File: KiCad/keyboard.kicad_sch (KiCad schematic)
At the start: 120 parts, among them J1 OLED_128x32, J2 Conn_01x02_Socket, J3 4P4C, J4 OLED_128x32, J5 Conn_01x02_Socket, J6 4P4C, SW1 Switch, SW2 SW_SPDT, SW3 Switch, SW4 SW_SPDT, U1 XIAO-HALF-HOLE-23P, U3 XIAO-HALF-HOLE-23P

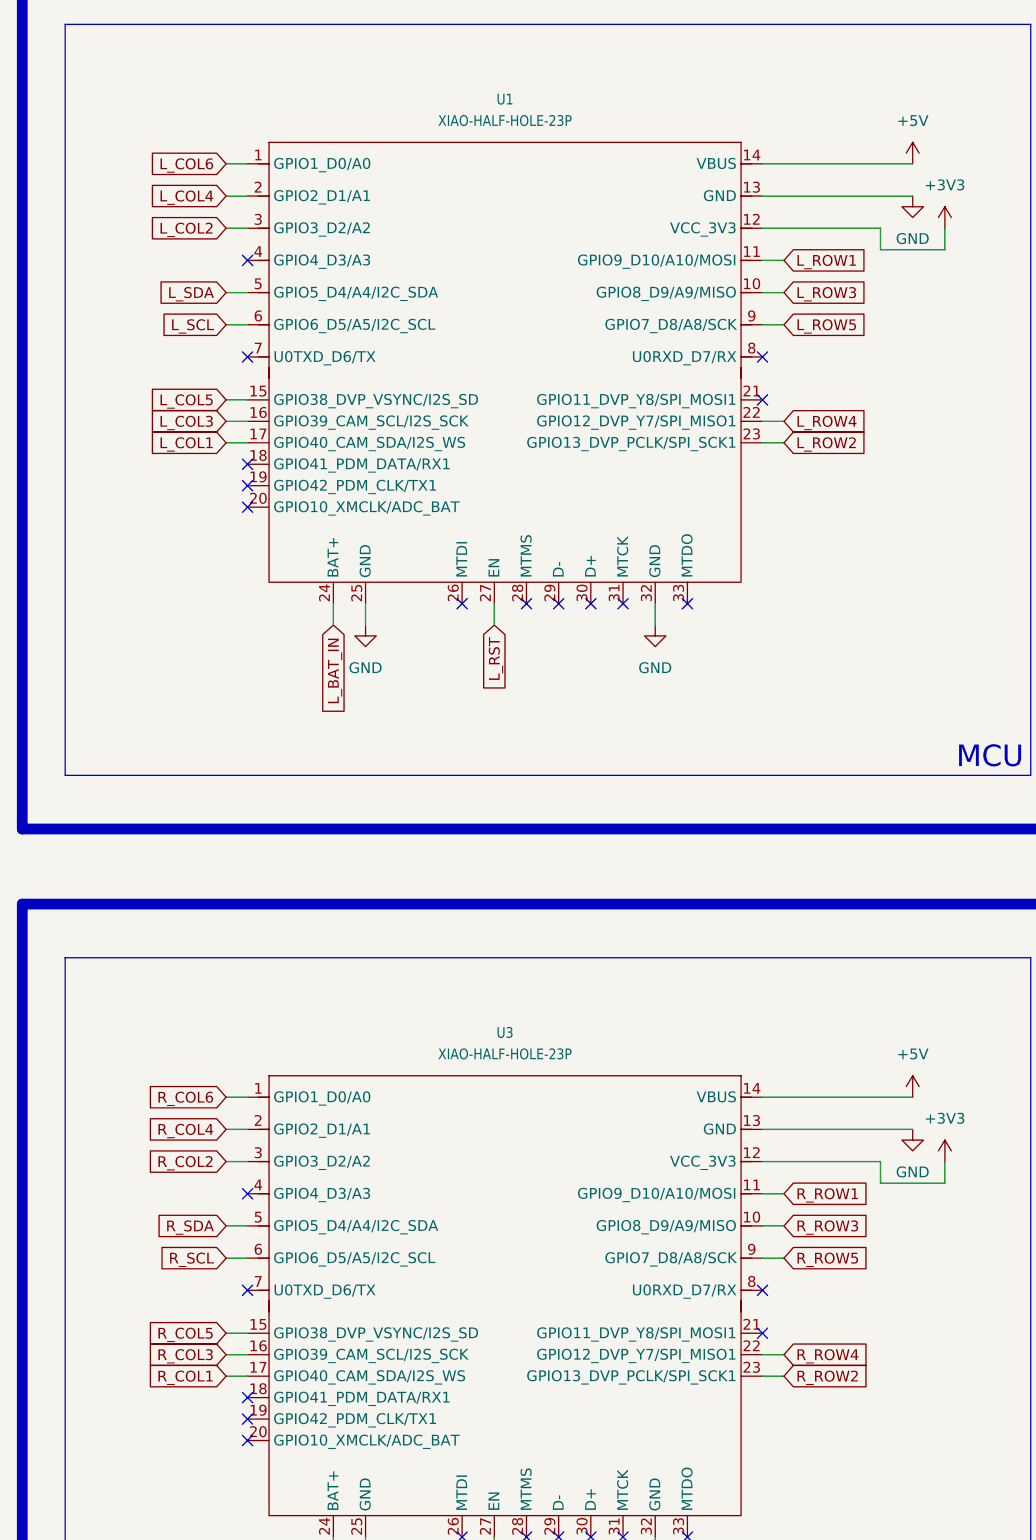
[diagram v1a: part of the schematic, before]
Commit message: PCB
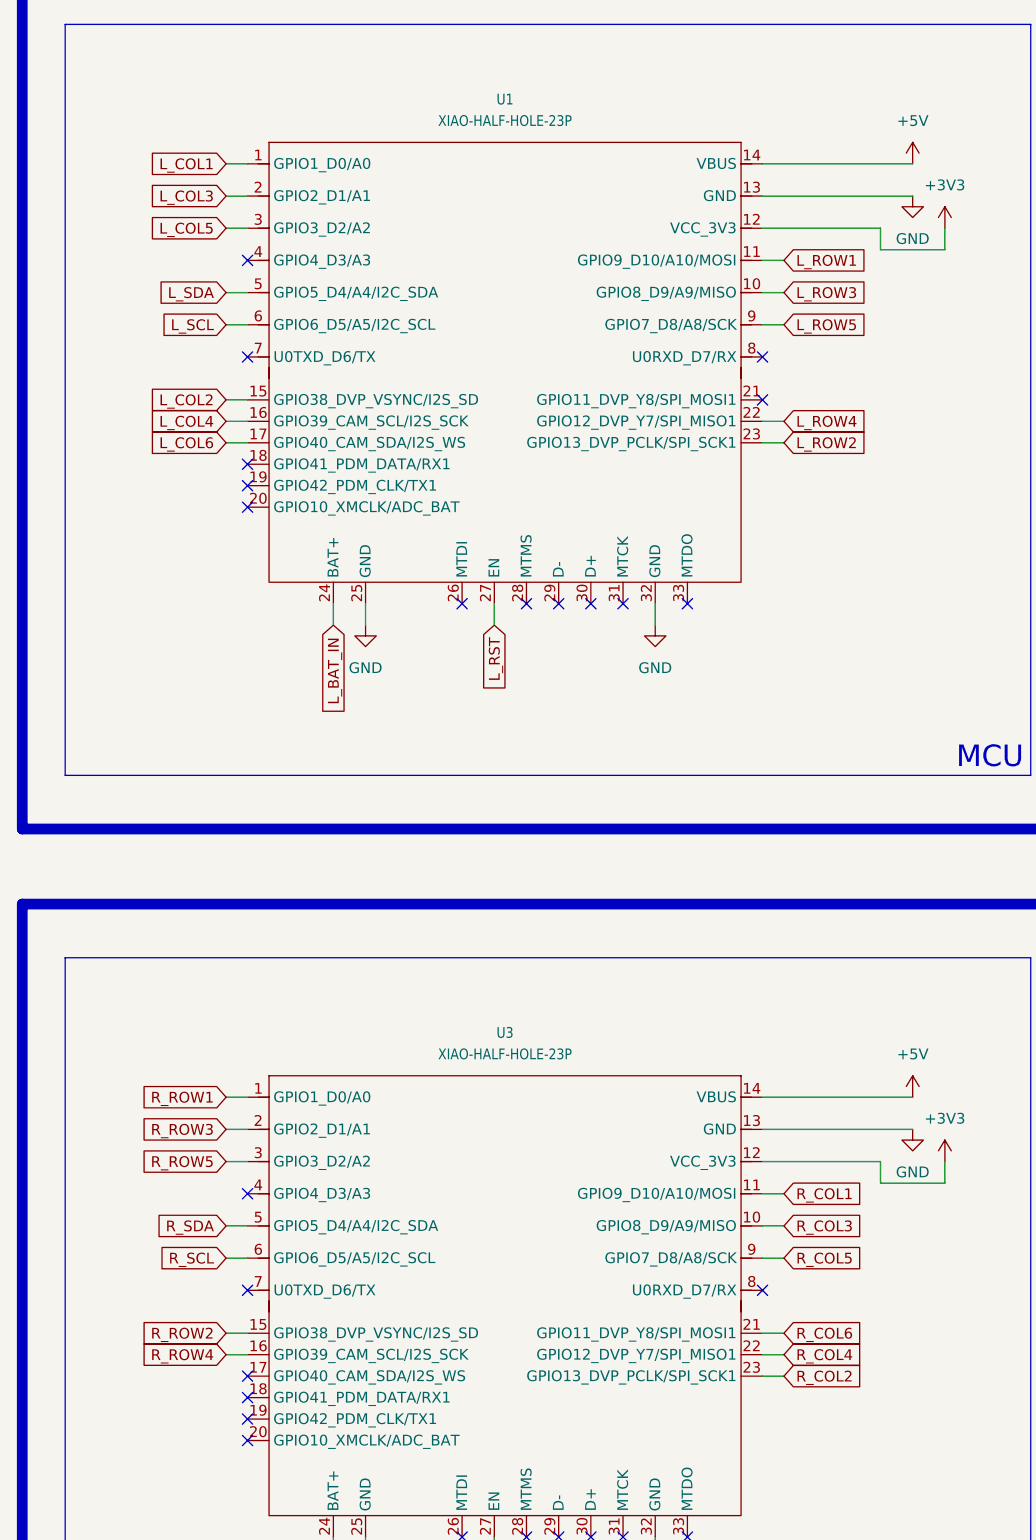
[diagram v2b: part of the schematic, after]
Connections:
- net L_COL1: now also U1.1 (GPIO1_D0/A0); no longer U1.17 (GPIO40_CAM_SDA/I2S_WS)
- net L_COL2: now also U1.15 (GPIO38_DVP_VSYNC/I2S_SD); no longer U1.3 (GPIO3_D2/A2)
- net L_COL3: now also U1.2 (GPIO2_D1/A1); no longer U1.16 (GPIO39_CAM_SCL/I2S_SCK)
- net L_COL4: now also U1.16 (GPIO39_CAM_SCL/I2S_SCK); no longer U1.2 (GPIO2_D1/A1)
- net L_COL5: now also U1.3 (GPIO3_D2/A2); no longer U1.15 (GPIO38_DVP_VSYNC/I2S_SD)
- net L_COL6: now also U1.17 (GPIO40_CAM_SDA/I2S_WS); no longer U1.1 (GPIO1_D0/A0)
- net R_COL1: now also U3.11 (GPIO9_D10/A10/MOSI); no longer U3.17 (GPIO40_CAM_SDA/I2S_WS)
- net R_COL2: now also U3.23 (GPIO13_DVP_PCLK/SPI_SCK1); no longer U3.3 (GPIO3_D2/A2)
- net R_COL3: now also U3.10 (GPIO8_D9/A9/MISO); no longer U3.16 (GPIO39_CAM_SCL/I2S_SCK)
- net R_COL4: now also U3.22 (GPIO12_DVP_Y7/SPI_MISO1); no longer U3.2 (GPIO2_D1/A1)
- net R_COL5: now also U3.9 (GPIO7_D8/A8/SCK); no longer U3.15 (GPIO38_DVP_VSYNC/I2S_SD)
- net R_COL6: now also U3.21 (GPIO11_DVP_Y8/SPI_MOSI1); no longer U3.1 (GPIO1_D0/A0)
- net R_ROW1: now also U3.1 (GPIO1_D0/A0); no longer U3.11 (GPIO9_D10/A10/MOSI)
- net R_ROW2: now also U3.15 (GPIO38_DVP_VSYNC/I2S_SD); no longer U3.23 (GPIO13_DVP_PCLK/SPI_SCK1)
- net R_ROW3: now also U3.2 (GPIO2_D1/A1); no longer U3.10 (GPIO8_D9/A9/MISO)
- net R_ROW4: now also U3.16 (GPIO39_CAM_SCL/I2S_SCK); no longer U3.22 (GPIO12_DVP_Y7/SPI_MISO1)
- net R_ROW5: now also U3.3 (GPIO3_D2/A2); no longer U3.9 (GPIO7_D8/A8/SCK)
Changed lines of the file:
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@@
 	)
 	(no_connect
-		(at 125.73 195.58)
-	)
-	(no_connect
 		(at 64.77 203.2)
 	)
@@
 	)
 	(no_connect
+		(at 64.77 200.66)
+	)
+	(no_connect
 		(at 64.77 208.28)
 	)
@@
 	(wire
 		(pts
-			(xy 62.23 200.66) (xy 64.77 200.66)
-		)
-		(stroke
-			(width 0)
-			(type default)
-		)
-	)
-	(wire
-		(pts
 			(xy 311.15 220.98) (xy 323.85 220.98)
 		)
@@
 	(wire
 		(pts
+			(xy 128.27 195.58) (xy 125.73 195.58)
+		)
+		(stroke
+			(width 0)
+			(type default)
+		)
+	)
+	(wire
+		(pts
 			(xy 280.67 172.72) (xy 280.67 185.42)
 		)
@@
 	(global_label "R_COL6"
 		(shape input)
-		(at 62.23 167.64 180)
+		(at 128.27 195.58 0)
 		(fields_autoplaced yes)
 		(effects
@@
 				(size 1.27 1.27)
 			)
-			(justify right)
+			(justify left)
 		)
 		(property "Intersheetrefs" "${INTERSHEET_REFS}"
-			(at 52.1691 167.64 0)
+			(at 138.3309 195.58 0)
 			(effects
 				(font
 					(size 1.27 1.27)
 				)
-				(justify right)
+				(justify left)
 				(hide yes)
 			)
@@
 	(global_label "L_COL5"
 		(shape input)
-		(at 62.23 85.09 180)
+		(at 62.23 64.77 180)
 		(fields_autoplaced yes)
 		(effects
@@
 		)
 		(property "Intersheetrefs" "${INTERSHEET_REFS}"
-			(at 52.411 85.09 0)
+			(at 52.411 64.77 0)
 			(effects
 				(font
@@
 	(global_label "R_COL3"
 		(shape input)
-		(at 62.23 198.12 180)
+		(at 128.27 182.88 0)
 		(fields_autoplaced yes)
 		(effects
@@
 				(size 1.27 1.27)
 			)
-			(justify right)
+			(justify left)
 		)
 		(property "Intersheetrefs" "${INTERSHEET_REFS}"
-			(at 52.1691 198.12 0)
+			(at 138.3309 182.88 0)
 			(effects
 				(font
 					(size 1.27 1.27)
 				)
-				(justify right)
+				(justify left)
 				(hide yes)
 			)
@@
 	(global_label "R_ROW2"
 		(shape input)
-		(at 128.27 200.66 0)
+		(at 62.23 195.58 180)
 		(fields_autoplaced yes)
 		(effects
@@
 				(size 1.27 1.27)
 			)
-			(justify left)
+			(justify right)
 		)
 		(property "Intersheetrefs" "${INTERSHEET_REFS}"
-			(at 138.7542 200.66 0)
+			(at 51.7458 195.58 0)
 			(effects
 				(font
 					(size 1.27 1.27)
 				)
-				(justify left)
+				(justify right)
 				(hide yes)
 			)
@@
 	(global_label "L_COL1"
 		(shape input)
-		(at 62.23 90.17 180)
+		(at 62.23 57.15 180)
 		(fields_autoplaced yes)
 		(effects
@@
 		)
 		(property "Intersheetrefs" "${INTERSHEET_REFS}"
-			(at 52.411 90.17 0)
+			(at 52.411 57.15 0)
 			(effects
 				(font
@@
 	(global_label "L_COL3"
 		(shape input)
-		(at 62.23 87.63 180)
+		(at 62.23 60.96 180)
 		(fields_autoplaced yes)
 		(effects
@@
 		)
 		(property "Intersheetrefs" "${INTERSHEET_REFS}"
-			(at 52.411 87.63 0)
+			(at 52.411 60.96 0)
 			(effects
 				(font
@@
 	(global_label "R_COL5"
 		(shape input)
-		(at 62.23 195.58 180)
+		(at 128.27 186.69 0)
 		(fields_autoplaced yes)
 		(effects
@@
 				(size 1.27 1.27)
 			)
-			(justify right)
+			(justify left)
 		)
 		(property "Intersheetrefs" "${INTERSHEET_REFS}"
-			(at 52.1691 195.58 0)
+			(at 138.3309 186.69 0)
 			(effects
 				(font
 					(size 1.27 1.27)
 				)
-				(justify right)
+				(justify left)
 				(hide yes)
 			)
@@
 	(global_label "R_COL2"
 		(shape input)
-		(at 62.23 175.26 180)
+		(at 128.27 200.66 0)
 		(fields_autoplaced yes)
 		(effects
@@
 				(size 1.27 1.27)
 			)
-			(justify right)
+			(justify left)
 		)
 		(property "Intersheetrefs" "${INTERSHEET_REFS}"
-			(at 52.1691 175.26 0)
+			(at 138.3309 200.66 0)
 			(effects
 				(font
 					(size 1.27 1.27)
 				)
-				(justify right)
+				(justify left)
 				(hide yes)
 			)
@@
 	(global_label "R_ROW4"
 		(shape input)
-		(at 128.27 198.12 0)
+		(at 62.23 198.12 180)
 		(fields_autoplaced yes)
 		(effects
@@
 				(size 1.27 1.27)
 			)
-			(justify left)
+			(justify right)
 		)
 		(property "Intersheetrefs" "${INTERSHEET_REFS}"
-			(at 138.7542 198.12 0)
+			(at 51.7458 198.12 0)
 			(effects
 				(font
 					(size 1.27 1.27)
 				)
-				(justify left)
+				(justify right)
 				(hide yes)
 			)
@@
 	(global_label "L_COL4"
 		(shape input)
-		(at 62.23 60.96 180)
+		(at 62.23 87.63 180)
 		(fields_autoplaced yes)
 		(effects
@@
 		)
 		(property "Intersheetrefs" "${INTERSHEET_REFS}"
-			(at 52.411 60.96 0)
+			(at 52.411 87.63 0)
 			(effects
 				(font
@@
 	(global_label "R_ROW3"
 		(shape input)
-		(at 128.27 182.88 0)
+		(at 62.23 171.45 180)
 		(fields_autoplaced yes)
 		(effects
@@
 				(size 1.27 1.27)
 			)
-			(justify left)
+			(justify right)
 		)
 		(property "Intersheetrefs" "${INTERSHEET_REFS}"
-			(at 138.7542 182.88 0)
+			(at 51.7458 171.45 0)
 			(effects
 				(font
 					(size 1.27 1.27)
 				)
-				(justify left)
+				(justify right)
 				(hide yes)
 			)
@@
 	(global_label "R_ROW5"
 		(shape input)
-		(at 128.27 186.69 0)
+		(at 62.23 175.26 180)
 		(fields_autoplaced yes)
 		(effects
@@
 				(size 1.27 1.27)
 			)
-			(justify left)
+			(justify right)
 		)
 		(property "Intersheetrefs" "${INTERSHEET_REFS}"
-			(at 138.7542 186.69 0)
+			(at 51.7458 175.26 0)
 			(effects
 				(font
 					(size 1.27 1.27)
 				)
-				(justify left)
+				(justify right)
 				(hide yes)
 			)
@@
 	(global_label "L_COL6"
 		(shape input)
-		(at 62.23 57.15 180)
+		(at 62.23 90.17 180)
 		(fields_autoplaced yes)
 		(effects
@@
 		)
 		(property "Intersheetrefs" "${INTERSHEET_REFS}"
-			(at 52.411 57.15 0)
+			(at 52.411 90.17 0)
 			(effects
 				(font
@@
 	(global_label "R_COL4"
 		(shape input)
-		(at 62.23 171.45 180)
+		(at 128.27 198.12 0)
 		(fields_autoplaced yes)
 		(effects
@@
 				(size 1.27 1.27)
 			)
-			(justify right)
+			(justify left)
 		)
 		(property "Intersheetrefs" "${INTERSHEET_REFS}"
-			(at 52.1691 171.45 0)
+			(at 138.3309 198.12 0)
 			(effects
 				(font
 					(size 1.27 1.27)
 				)
-				(justify right)
+				(justify left)
 				(hide yes)
 			)
@@
 	(global_label "R_ROW1"
 		(shape input)
-		(at 128.27 179.07 0)
+		(at 62.23 167.64 180)
 		(fields_autoplaced yes)
 		(effects
@@
 				(size 1.27 1.27)
 			)
-			(justify left)
+			(justify right)
 		)
 		(property "Intersheetrefs" "${INTERSHEET_REFS}"
-			(at 138.7542 179.07 0)
+			(at 51.7458 167.64 0)
 			(effects
 				(font
 					(size 1.27 1.27)
 				)
-				(justify left)
+				(justify right)
 				(hide yes)
 			)
@@
 	(global_label "L_COL2"
 		(shape input)
-		(at 62.23 64.77 180)
+		(at 62.23 85.09 180)
 		(fields_autoplaced yes)
 		(effects
@@
 		)
 		(property "Intersheetrefs" "${INTERSHEET_REFS}"
-			(at 52.411 64.77 0)
+			(at 52.411 85.09 0)
 			(effects
 				(font
@@
 	(global_label "R_COL1"
 		(shape input)
-		(at 62.23 200.66 180)
+		(at 128.27 179.07 0)
 		(fields_autoplaced yes)
 		(effects
@@
 				(size 1.27 1.27)
 			)
-			(justify right)
+			(justify left)
 		)
 		(property "Intersheetrefs" "${INTERSHEET_REFS}"
-			(at 52.1691 200.66 0)
+			(at 138.3309 179.07 0)
 			(effects
 				(font
 					(size 1.27 1.27)
 				)
-				(justify right)
+				(justify left)
 				(hide yes)
 			)

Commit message: partially update pt2
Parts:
- J3, J6: footprint Connector_RJ:RJ9_Evercom_5301-440xxx_Horizontal -> chinh4thepro:RJ9_Evercom_5301-440xxx_Horizontal
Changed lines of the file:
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@@
 			)
 		)
-		(property "Footprint" "Connector_RJ:RJ9_Evercom_5301-440xxx_Horizontal"
+		(property "Footprint" "chinh4thepro:RJ9_Evercom_5301-440xxx_Horizontal"
 			(at 194.31 194.31 90)
 			(effects
@@
 			)
 		)
-		(property "Footprint" "Connector_RJ:RJ9_Evercom_5301-440xxx_Horizontal"
+		(property "Footprint" "chinh4thepro:RJ9_Evercom_5301-440xxx_Horizontal"
 			(at 194.31 83.82 90)
 			(effects
